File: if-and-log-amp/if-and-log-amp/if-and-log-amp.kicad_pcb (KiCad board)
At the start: 2 copper layers, 91.7 x 48.8 mm, 74 parts, among them J301 Coax, J305 Conn_01x03, J306 Conn_01x02, J307 Conn_Coaxial, Q301 2N3904, T301 FT37-43 8:2 t, U301 AD603AQ, U302 L78L05_TO92, U303 LM317L_TO92, U304 AD8307AN, U305 CA3140

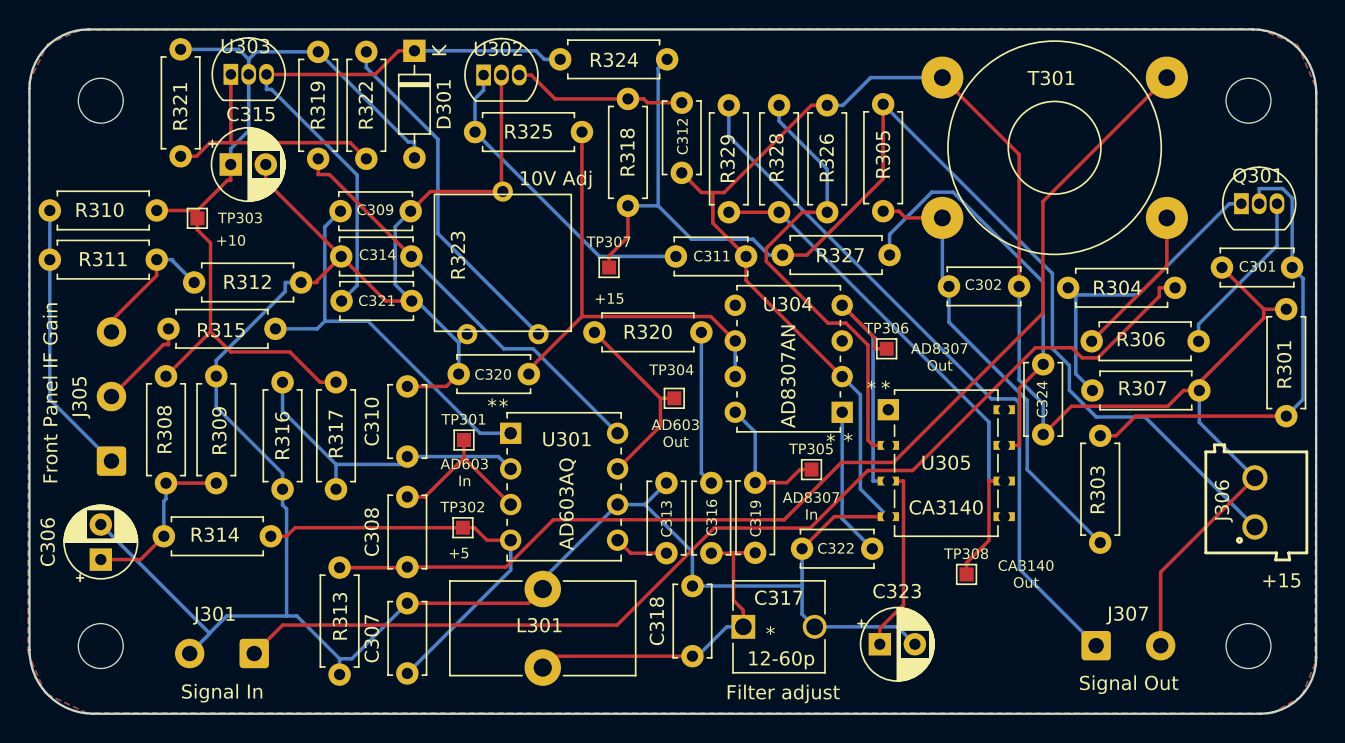
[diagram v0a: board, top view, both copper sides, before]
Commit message: IF Log Amp V2
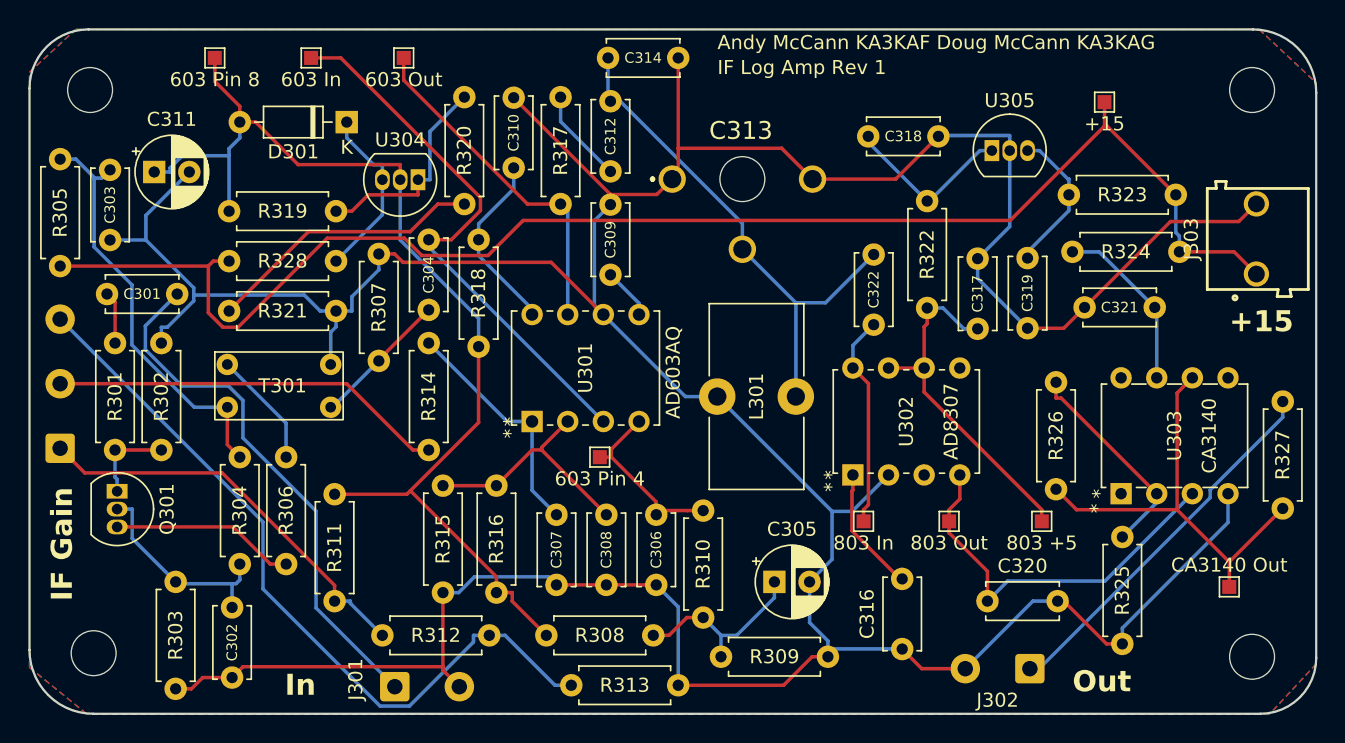
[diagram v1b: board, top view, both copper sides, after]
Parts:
- removed C315: 22u, Capacitor_THT:CP_Radial_D5.0mm_P2.50mm
- removed C323: .001u, Capacitor_THT:CP_Radial_D5.0mm_P2.50mm
- removed C324: .1u, Capacitor_THT:C_Disc_D5.0mm_W2.5mm_P5.00mm
- removed J305: Conn_01x03, Connector_Wire:SolderWire-0.5sqmm_1x03_P4.6mm_D0.9mm_OD2.1mm
- removed J306: Conn_01x02, if-log-amp:691103110002
- removed J307: Conn_Coaxial, Connector_Wire:SolderWire-0.5sqmm_1x02_P4.6mm_D0.9mm_OD2.1mm
- removed R329: 1k, Resistor_THT:R_Axial_DIN0207_L6.3mm_D2.5mm_P7.62mm_Horizontal
- added C303: .1u, Capacitor_THT:C_Disc_D5.0mm_W2.5mm_P5.00mm, F.Cu at (101.1, 90.4)
- added C304: .01u, Capacitor_THT:C_Disc_D5.0mm_W2.5mm_P5.00mm, F.Cu at (123.8, 100.4)
- added C305: 100u, Capacitor_THT:CP_Radial_D5.0mm_P2.50mm, F.Cu at (148.4, 119.8)
- added J302: Conn_Coaxial, Connector_Wire:SolderWire-0.5sqmm_1x02_P4.6mm_D0.9mm_OD2.1mm, F.Cu at (166.6, 126.0)
- added J303: +15 In, spectrum analyzer:691103110002, F.Cu at (182.8, 95.3)
- added J304: Conn_01x03, Connector_Wire:SolderWire-0.5sqmm_1x03_P4.6mm_D0.9mm_OD2.1mm, F.Cu at (97.5, 110.3)
- added R302: 470, Resistor_THT:R_Axial_DIN0207_L6.3mm_D2.5mm_P7.62mm_Horizontal, F.Cu at (104.7, 110.4)
- added TP309: 803 +5, TestPoint:TestPoint_Pad_1.0x1.0mm, F.Cu at (167.5, 115.5)
- C306: value 100u -> .1u; footprint Capacitor_THT:CP_Radial_D5.0mm_P2.50mm -> Capacitor_THT:C_Disc_D5.0mm_W2.5mm_P5.00mm
- C308: value .01u -> .1u
- C309: value .1u -> 18p
- C311: value .1u -> 22u; footprint Capacitor_THT:C_Disc_D5.0mm_W2.5mm_P5.00mm -> Capacitor_THT:CP_Radial_D5.0mm_P2.50mm
- C312: value .22u -> 5.6p
- C313: value 18p -> 5-65pf; footprint Capacitor_THT:C_Disc_D5.0mm_W2.5mm_P5.00mm -> spectrum analyzer:BFC280831659
- C314: value .1u -> 220p
- C316: value 5.6p -> .1u
- C317: value 12-60p -> .1u; footprint if-log-amp:GKG60015 -> Capacitor_THT:C_Disc_D5.0mm_W2.5mm_P5.00mm
- C318: value 180p -> .1u
- C319: value 5.6p -> .22u
- C320: value .1u -> .001u
- C322: value .1u -> 5.6p
- D301: value 1N4150 -> 1N4148
- R301: value 2k -> 47
- R303: value 10k -> 2k
- R304: value 47 -> 10k
- R307: value 470 -> 100
- R310: value 680 -> 51
- R311: value 510 -> 680
- R312: value 1k -> 510
- R313: value 100 -> 1k
- R314: value 51 -> 2.2k
- R315: value 2.2k -> 5.6k
- R316: value 5.6k -> 4.3k
- R317: value 4.3k -> 1k
- R319: value 10 -> 220
- R320: value 1k -> 1.5k
- R321: value 220 -> 82
- R322: value 1.5k -> 10
- R323: value 100 -> 10; footprint if-log-amp:Potentiometer_Bourns_3386G_Vertical -> Resistor_THT:R_Axial_DIN0207_L6.3mm_D2.5mm_P7.62mm_Horizontal
- R324: value 10 -> 51
- R325: value 10 -> 680
- R326: value 680 -> 2.2k
- R327: value 51 -> 1k
- R328: value 2.2k -> 10
- T301: footprint Transformer_THT:Transformer_Toroid_Horizontal_D14.0mm_Amidon-T50 -> spectrum analyzer:Transformer Vertical 1P 1S
- TP301: value TestPoint -> 603 In
- TP302: value TestPoint -> 603 Pin 4
- TP303: value TestPoint -> 603 Pin 8
- TP304: value TestPoint -> 603 Out
- TP305: value TestPoint -> 803 In
- TP306: value TestPoint -> 803 Out
- TP307: value TestPoint -> +15
- TP308: value TestPoint -> CA3140 Out
- U301: footprint if-log-amp:AD603AQ -> spectrum analyzer:AD603AQ
- U302: value L78L05_TO92 -> AD8307; footprint Package_TO_SOT_THT:TO-92_Inline -> spectrum analyzer:AD8307AN
- U303: value LM317L_TO92 -> CA3140; footprint Package_TO_SOT_THT:TO-92_Inline -> spectrum analyzer:CA3140EZ
- U304: value AD8307AN -> LM317L_TO92; footprint if-log-amp:AD8307AN -> Package_TO_SOT_THT:TO-92_Inline
- U305: value CA3140 -> L78L05_TO92; footprint if-log-amp:CA3140EZ -> Package_TO_SOT_THT:TO-92_Inline
- moved H303 91.2 mm to (99.9, 124.9)
- moved R301 83.5 mm to (101.4, 110.4)
- moved Q301 82.7 mm to (101.6, 113.3), turned to -90 degrees
- moved H302 82.0 mm to (182.5, 84.7)
- moved C301 74.5 mm to (105.9, 99.3), turned to 180 degrees
- moved U303 70.1 mm to (173.1, 113.5), turned to 90 degrees
- moved R303 65.9 mm to (105.8, 119.8), turned to -90 degrees
- moved R304 60.2 mm to (110.3, 110.9), turned to -90 degrees
- moved R305 59.8 mm to (97.5, 97.3), turned to 90 degrees
- moved R306 58.0 mm to (113.6, 110.9), turned to -90 degrees
- moved C302 56.0 mm to (109.8, 121.6), turned to -90 degrees
- moved R325 54.4 mm to (173.2, 116.6), turned to -90 degrees
- moved C321 52.9 mm to (170.5, 100.2)
- moved R307 50.9 mm to (120.2, 104.0), turned to 90 degrees
- moved R310 48.6 mm to (143.4, 122.3), turned to 90 degrees
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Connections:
- C301 pad 1: GND -> Net-(J301-In)
- C302 pad 1: Net-(C302-Pad1) -> Net-(Q301-B)
- C306 pad 1: Net-(C306-Pad1) -> Net-(U301-COMM)
- C307 pad 1: Net-(C307-Pad1) -> Net-(U301-GPOS)
- C308 pad 1: Net-(C308-Pad1) -> Net-(U301-GNEG)
- C308 pad 2: Net-(C308-Pad2) -> GND
- C309 pad 1: Net-(C309-Pad1) -> Net-(U301-FDBK)
- C310 pad 1: Net-(C310-Pad1) -> GND
- C310 pad 2: GND -> Net-(U301-VPOS)
- C311 pad 1: /+5 -> /+10
- C312 pad 2: GND -> Net-(C312-Pad2)
- C313 pad 1: Net-(C313-Pad1) -> GND
- C313 pad 2: GND -> Net-(C312-Pad2)
- C314 pad 1: GND -> Net-(C312-Pad2)
- C314 pad 2: Net-(C314-Pad2) -> GND
- C316 pad 1: Net-(C316-Pad1) -> GND
- C316 pad 2: Net-(C316-Pad2) -> Net-(U302-INM)
- C317 pad 1: Net-(C316-Pad2) -> Net-(U302-ENB)
- C318 pad 1: Net-(C316-Pad2) -> /+5
- C319 pad 1: Net-(C316-Pad2) -> Net-(U305-VI)
- C319 pad 2: Net-(C319-Pad2) -> GND
- C320 pad 1: Net-(C320-Pad1) -> Net-(U302-OUT)
- C321 pad 1: Net-(C321-Pad1) -> GND
- C321 pad 2: GND -> Net-(U303-V+)
- C322 pad 1: GND -> Net-(C312-Pad2)
- C322 pad 2: Net-(C322-Pad2) -> Net-(U302-INP)
- D301 pad 1: Net-(C321-Pad1) -> Net-(D301-K)
- J301 pad 1: /In -> Net-(J301-In)
- L301 pad 2: Net-(C316-Pad2) -> Net-(C312-Pad2)
- Q301 pad 1: Net-(Q301-Pad1) -> Net-(Q301-E)
- Q301 pad 2: Net-(C301-Pad2) -> Net-(Q301-B)
- R301 pad 1: Net-(C301-Pad2) -> Net-(Q301-E)
- R301 pad 2: GND -> Net-(C301-Pad2)
- R303 pad 1: Net-(C302-Pad1) -> Net-(Q301-B)
- R303 pad 2: Net-(C301-Pad2) -> GND
- R304 pad 1: Net-(Q301-Pad1) -> Net-(T301-AA)
- R304 pad 2: /In -> Net-(Q301-B)
- R305 pad 2: Net-(C302-Pad1) -> Net-(T301-AA)
- R306 pad 1: Net-(R306-Pad1) -> Net-(T301-AB)
- R307 pad 1: Net-(Q301-Pad1) -> Net-(T301-SB)
- R308 pad 2: Net-(C306-Pad1) -> Net-(C305-Pad1)
- R309 pad 1: Net-(C306-Pad1) -> Net-(C305-Pad1)
- R310 pad 1: /+10 -> Net-(C305-Pad1)
- R310 pad 2: Net-(C303-Pad3) -> Net-(U301-COMM)
- R311 pad 1: Net-(C303-Pad3) -> /+10
- R312 pad 2: GND -> Net-(J304-Pin_3)
- R313 pad 1: Net-(C308-Pad1) -> Net-(J304-Pin_3)
- R314 pad 1: Net-(C306-Pad1) -> Net-(U301-GPOS)
- R314 pad 2: Net-(C307-Pad1) -> Net-(J304-Pin_2)
- R315 pad 1: Net-(C309-Pad1) -> Net-(U301-GNEG)
- R315 pad 2: Net-(C304-Pad3) -> GND
- R316 pad 1: Net-(C310-Pad1) -> Net-(U301-GNEG)
- R316 pad 2: GND -> /+10
- R317 pad 1: Net-(C310-Pad1) -> Net-(U301-VOUT)
- R317 pad 2: /+10 -> Net-(C312-Pad1)
- R318 pad 1: /+15 -> /+10
- R318 pad 2: Net-(C312-Pad1) -> Net-(U301-VPOS)
- R319 pad 2: Net-(C314-Pad2) -> Net-(U304-ADJ)
- R320 pad 1: Net-(R320-Pad1) -> Net-(U304-ADJ)
- R320 pad 2: Net-(C316-Pad1) -> Net-(R320-Pad2)
- R321 pad 1: /+10 -> Net-(R320-Pad2)
- R321 pad 2: Net-(R321-Pad2) -> GND
- R322 pad 1: Net-(R321-Pad2) -> /+5
- R322 pad 2: Net-(R322-Pad2) -> Net-(U302-ENB)
- R323 pad 1: Net-(R322-Pad2) -> /+15
- R323 pad 2: GND -> Net-(U305-VI)
- R324 pad 1: /+15 -> Net-(U303-V+)
- R324 pad 2: Net-(C321-Pad1) -> /+15
- R325 pad 1: /+5 -> Net-(U303--)
- R325 pad 2: Net-(C320-Pad1) -> GND
- R326 pad 2: GND -> Net-(U303--)
- R327 pad 1: Net-(C324-Pad2) -> Net-(R326-Pad1)
- R327 pad 2: /+15 -> Net-(J302-In)
- R328 pad 1: Net-(R328-Pad1) -> Net-(D301-K)
- R328 pad 2: Net-(R326-Pad1) -> /+15
- T301 pad 1: Net-(C302-Pad1) -> Net-(T301-AA)
- T301 pad 2: Net-(R306-Pad1) -> Net-(T301-SB)
- T301 pad 3: GND -> Net-(T301-AB)
- T301 pad 4: Net-(C308-Pad1) -> GND
- TP301 pad 1: Net-(C308-Pad2) -> Net-(U301-VINP)
- TP302 pad 1: Net-(C307-Pad1) -> Net-(U301-COMM)
- TP304 pad 1: Net-(R320-Pad1) -> Net-(U301-VOUT)
- TP305 pad 1: Net-(C319-Pad2) -> Net-(U302-INP)
- TP306 pad 1: Net-(C323-Pad1) -> Net-(U302-OUT)
- TP308 pad 1: Net-(R328-Pad1) -> Net-(R326-Pad1)
- U301 pad 1: Net-(C309-Pad1) -> Net-(U301-GPOS)
- U301 pad 2: Net-(C310-Pad1) -> Net-(U301-GNEG)
- U301 pad 3: Net-(C308-Pad2) -> Net-(U301-VINP)
- U301 pad 4: Net-(C307-Pad1) -> Net-(U301-COMM)
- U301 pad 5: Net-(C313-Pad1) -> Net-(U301-FDBK)
- U301 pad 7: Net-(R320-Pad1) -> Net-(U301-VOUT)
- U301 pad 8: Net-(C314-Pad2) -> Net-(U301-VPOS)
- U302 pad 1: /+5 -> Net-(U302-INM)
- U302 pad 3: Net-(C312-Pad1) -> unconnected-(U302-OFS-Pad3)
- U303 pad 1: Net-(R321-Pad2) -> unconnected-(U303-NULL-Pad1)
- U303 pad 2: /+10 -> Net-(U303--)
- U303 pad 3: Net-(C321-Pad1) -> Net-(U302-OUT)
- U304 pad 1: Net-(C322-Pad2) -> Net-(U304-ADJ)
- U304 pad 2: GND -> /+10
- U304 pad 3: unconnected-(U304-Pad3) -> Net-(D301-K)
- U305 pad 1: unconnected-(U305-Pad1) -> /+5
- U305 pad 2: Net-(R326-Pad1) -> GND
- U305 pad 3: Net-(C323-Pad1) -> Net-(U305-VI)
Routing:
- net Net-(C308-Pad1): track 78.1 -> 0.00 mm
- net /In: track 77.4 -> 0.00 mm
- net Net-(J304-Pin_3): track 0.00 -> 54.5 mm
- net Net-(C325-Pad1): track 50.3 -> 0.00 mm
- net Net-(C321-Pad1): track 41.4 -> 0.00 mm
- net Net-(U301-VINP): track 0.00 -> 39.8 mm
- net Net-(R328-Pad1): track 38.4 -> 0.00 mm
- net Net-(J301-In): track 0.00 -> 38.2 mm
- net Net-(C312-Pad2): track 0.00 -> 37.0 mm
- net Net-(C320-Pad1): track 33.0 -> 0.00 mm
- net Net-(C323-Pad1): track 32.8 -> 0.00 mm
- net Net-(C302-Pad1): track 32.2 -> 0.00 mm
- net Net-(C307-Pad1): track 30.3 -> 0.00 mm
- net Net-(C301-Pad2): track 33.9 -> 3.73 mm
- net Net-(C314-Pad2): track 30.1 -> 0.00 mm
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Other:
- board text added: "IF Gain"
- board text added: "IF Log Amp Rev 1"
- board text added: "In"
- board text added: "Out"
- board text removed: "+10"
- board text removed: "+5"
- board text removed: "10V Adj"
- board text removed: "AD603 In"
- board text removed: "AD603 Out"
- board text removed: "AD8307 In"
- board text removed: "AD8307 Out"
- board text removed: "CA3140 Out"
- board text removed: "Filter adjust"
- board text removed: "Front Panel IF Gain"
- board text removed: "Signal In"
- board text removed: "Signal Out"
- board text removed: "Spectrum Analyzer IF and Log Amp Board Rev 1.0"
